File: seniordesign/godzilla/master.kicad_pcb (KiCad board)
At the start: 2 copper layers, 83.8 x 124.5 mm, 117 parts, among them CON1 USB-MICRO-B, IC1 ATTINY24-SS, J1 USB, P1 GND, P1 JTAG_PROG, P1 PROG_PINS, P1 SERVO_PWMS, P2 BATT+, P2 GPIO, P2 UART_PROG, P3 OUT, P3 ULTRA_FRONT, P4 ULTRA_BACK, Q1 BC847S, Q2 BC847S, SW1 DIPS_04, SW2 SW_PUSH, U1 ADP151AUJZ-3.3-R7, U1 FT234XD, U1 TPS62133, U2 MSP430G2153, U2 TM4C123GH6PM, U3 ADP151AUJZ-3.3-R7, U3 RN-42, U4 FGPMMOPA6H, U5 SN74LV1T04, U6 SN74LV1T04, X1 16.00 MHz

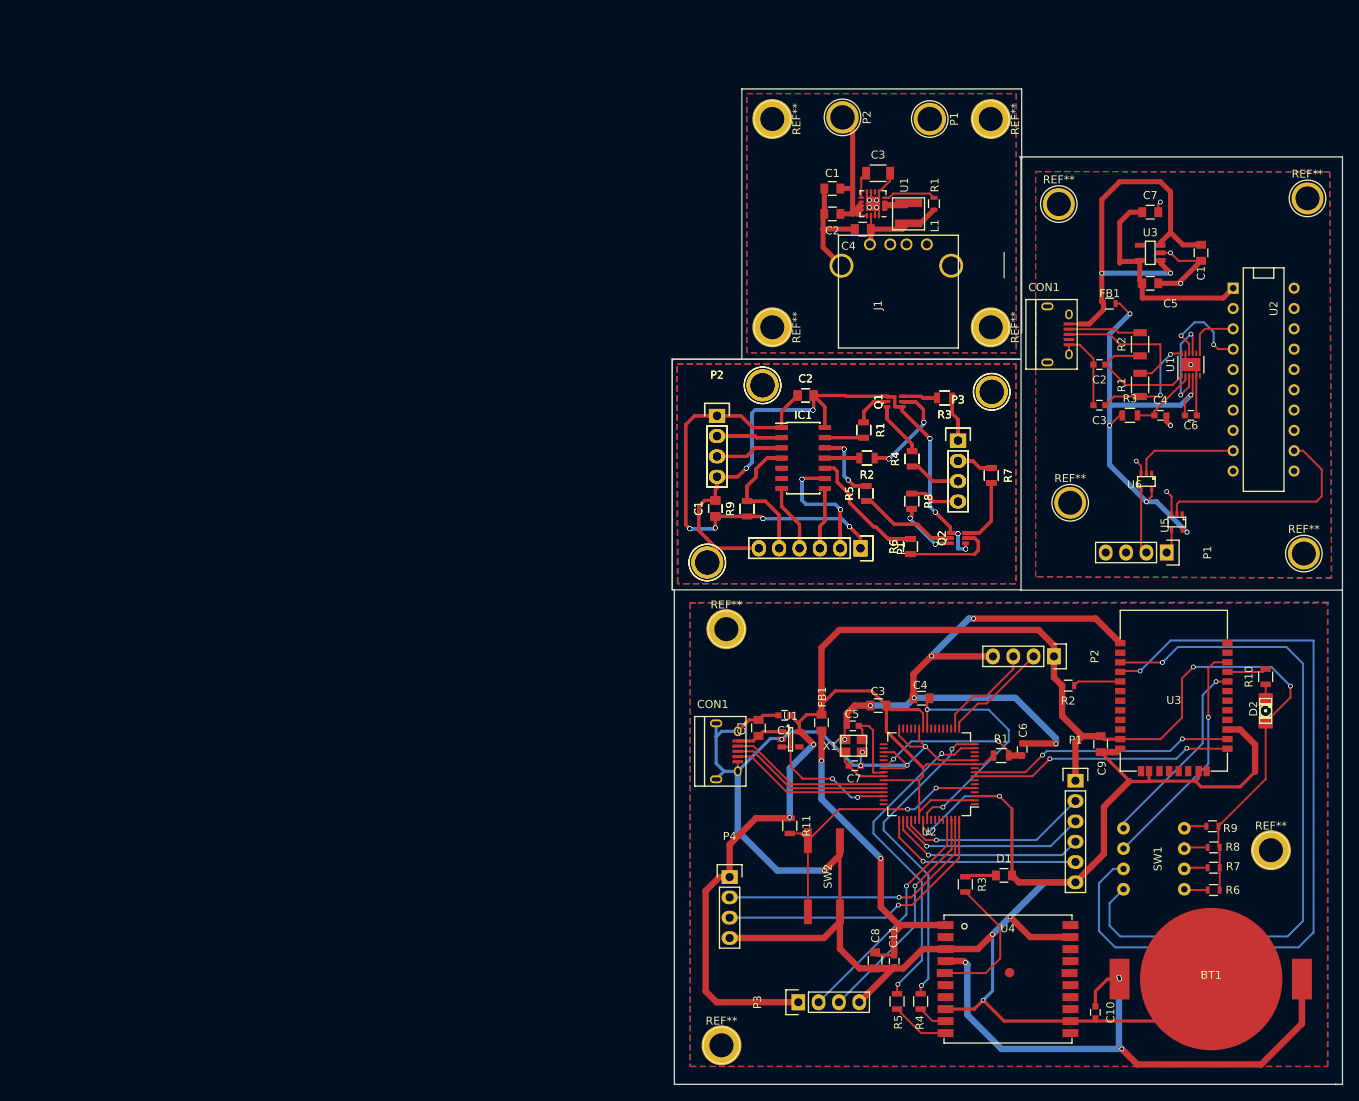
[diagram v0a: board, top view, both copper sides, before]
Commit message: Save Gerber files ,revision 9
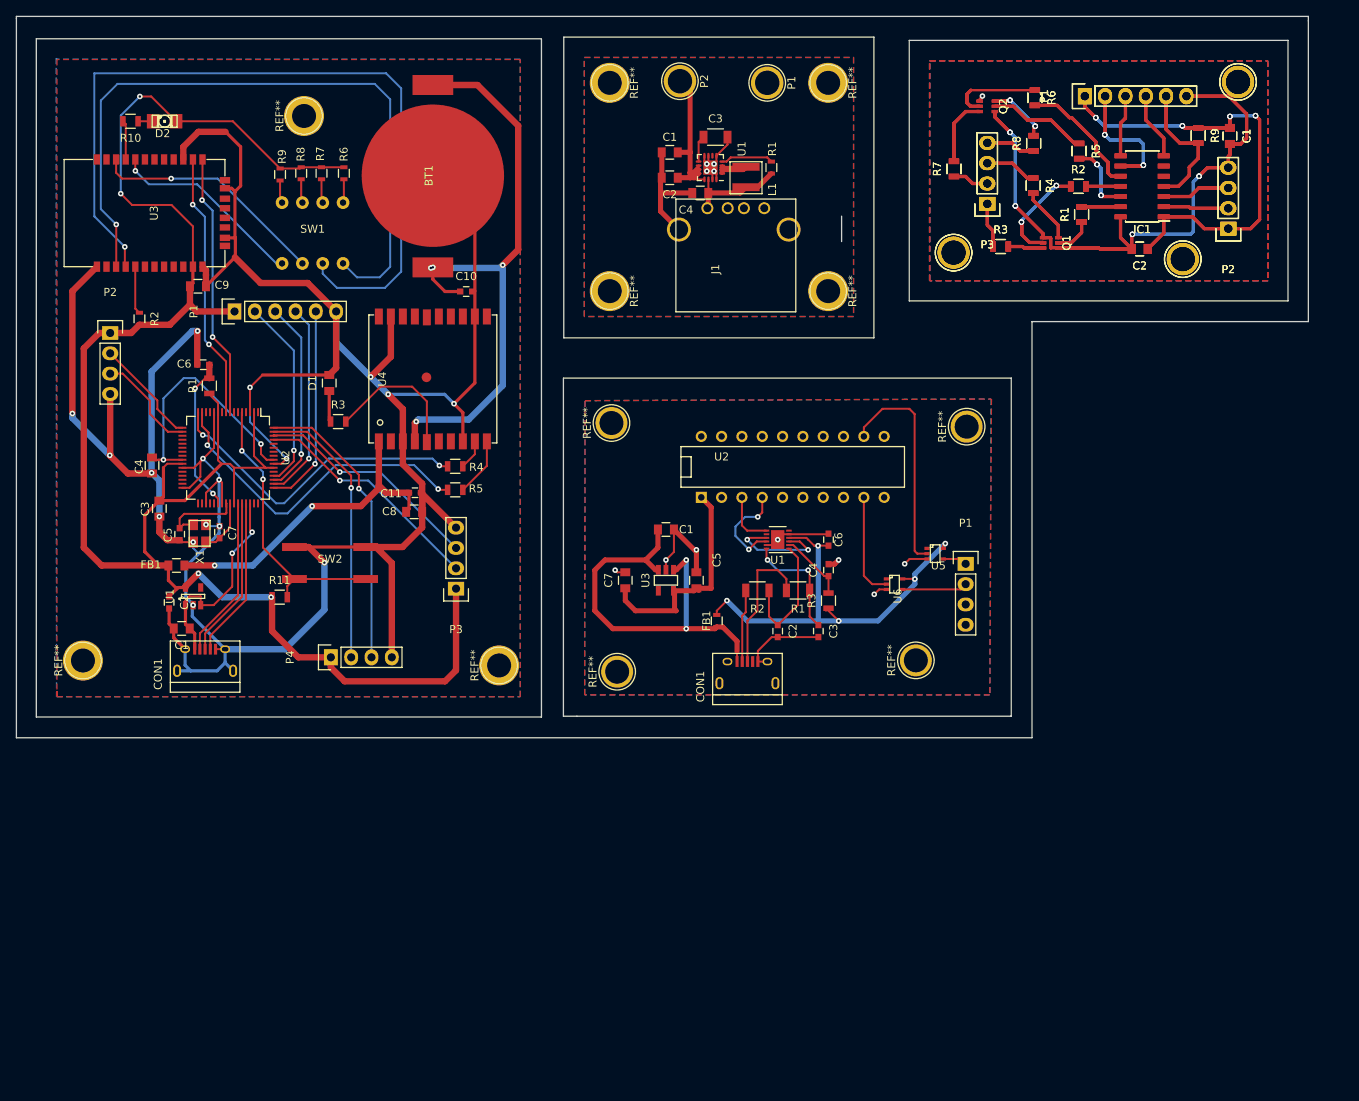
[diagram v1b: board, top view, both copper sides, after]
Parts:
- removed the C1 at (144.0, 99.5) (x2)
- removed the C2 at (155.3, 85.3) (x2)
- removed the IC1 at (155.0, 93.2) (x2)
- removed the P1 at (162.2, 104.4) (x2)
- removed the P2 at (144.2, 87.9) (x2)
- removed the P3 at (174.3, 91.0) (x2)
- removed the Q1 at (166.4, 86.1) (x2)
- removed the Q2 at (174.3, 103.2) (x2)
- removed the R1 at (162.6, 89.7) (x2)
- removed the R2 at (163.0, 93.2) (x2)
- removed the R3 at (172.7, 85.6) (x2)
- removed the R4 at (168.6, 93.3) (x2)
- removed the R5 at (162.9, 97.6) (x2)
- removed the R6 at (168.4, 104.2) (x2)
- removed the R7 at (178.5, 95.4) (x2)
- removed the R8 at (168.6, 98.6) (x2)
- removed the R9 at (148.0, 99.5) (x2)
- removed the REF** at (143.0, 106.2) (x2)
- removed the REF** at (178.6, 84.9) (x2)
- removed the REF** at (149.9, 84.1) (x2)
- added C1 (x2): 10u, Capacitors_SMD:C_0805, F.Cu at (208.3, 52.9)
- added C2 (x2): 0.1u, Capacitors_SMD:C_0805, F.Cu at (197.1, 67.0)
- added IC1 (x2): ATTINY24-SS, Housings_SOIC:SOIC-14_3.9x8.7mm_Pitch1.27mm, F.Cu at (197.4, 59.2)
- added P1 (x2): PROG_PINS, Pin_Headers:Pin_Header_Straight_1x06, F.Cu at (190.2, 47.9)
- added P2 (x2): GPIO, Pin_Headers:Pin_Header_Straight_1x04, F.Cu at (208.1, 64.5)
- added P3 (x2): OUT, Pin_Headers:Pin_Header_Straight_1x04, F.Cu at (178.0, 61.4)
- added Q1 (x2): BC847S, custom_footprints:SOT-363, F.Cu at (185.9, 66.3)
- added Q2 (x2): BC847S, custom_footprints:SOT-363, F.Cu at (178.0, 49.2)
- added R1 (x2): 0, Resistors_SMD:R_0805, F.Cu at (189.8, 62.7)
- added R2 (x2): 0, Resistors_SMD:R_0805, F.Cu at (189.4, 59.2)
- added R3 (x2): 90, Resistors_SMD:R_0805, F.Cu at (179.7, 66.7)
- added R4 (x2): 90, Resistors_SMD:R_0805, F.Cu at (183.7, 59.1)
- added R5 (x2): 0, Resistors_SMD:R_0805, F.Cu at (189.5, 54.8)
- added R6 (x2): 0, Resistors_SMD:R_0805, F.Cu at (184.0, 48.1)
- added R7 (x2): 90, Resistors_SMD:R_0805, F.Cu at (173.8, 57.0)
- added R8 (x2): 90, Resistors_SMD:R_0805, F.Cu at (183.8, 53.8)
- added R9 (x2): 33k, Resistors_SMD:R_0805, F.Cu at (204.4, 52.9)
- added REF** (x2): 1pin, Connect:1pin, F.Cu at (209.4, 46.2)
- added REF** (x2): 1pin, Connect:1pin, F.Cu at (173.8, 67.5)
- added REF** (x2): 1pin, Connect:1pin, F.Cu at (202.4, 68.3)
- moved R10 158.0 mm to (70.9, 51.1), turned to 180 degrees
- moved D2 156.1 mm to (75.2, 51.1), turned to 180 degrees
- moved REF** 151.8 mm to (92.6, 50.4), turned to 90 degrees
- moved R9 142.2 mm to (89.6, 57.7), turned to 270 degrees
- moved R8 141.8 mm to (92.2, 57.6), turned to 270 degrees
- moved R7 141.3 mm to (94.8, 57.6), turned to 270 degrees
- moved U3 141.3 mm to (73.9, 62.5), turned to 90 degrees
- moved R6 140.9 mm to (97.6, 57.6), turned to 270 degrees
- moved BT1 139.8 mm to (108.7, 57.9), turned to 270 degrees
- moved SW1 131.1 mm to (93.7, 65.0), turned to 180 degrees
- moved C9 126.5 mm to (79.3, 71.7), turned to 0 degrees
- moved R2 124.8 mm to (72.0, 75.8), turned to 270 degrees
- moved P2 124.7 mm to (68.4, 77.5), turned to 0 degrees
- moved P1 120.4 mm to (83.9, 74.8), turned to 90 degrees
- moved C10 119.6 mm to (112.9, 72.4), turned to 0 degrees
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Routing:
- net GND: track 609.3 -> 601.1 mm, vias 40 -> 37
- net +5V: track 169.2 -> 167.8 mm
- net Net-(C1-Pad1): track 98.5 -> 99.2 mm
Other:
- board size 83.8 x 124.5 mm -> 161.5 x 90.2 mm
- net class Default: via_dia 0.6 -> 0.7; via_drill 0.4 -> 0.3
- net class Power: via_dia 0.6 -> 0.7; via_drill 0.4 -> 0.3
